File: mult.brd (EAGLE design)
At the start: 100 x 80 mm, 18 parts, among them IC1 TL074P

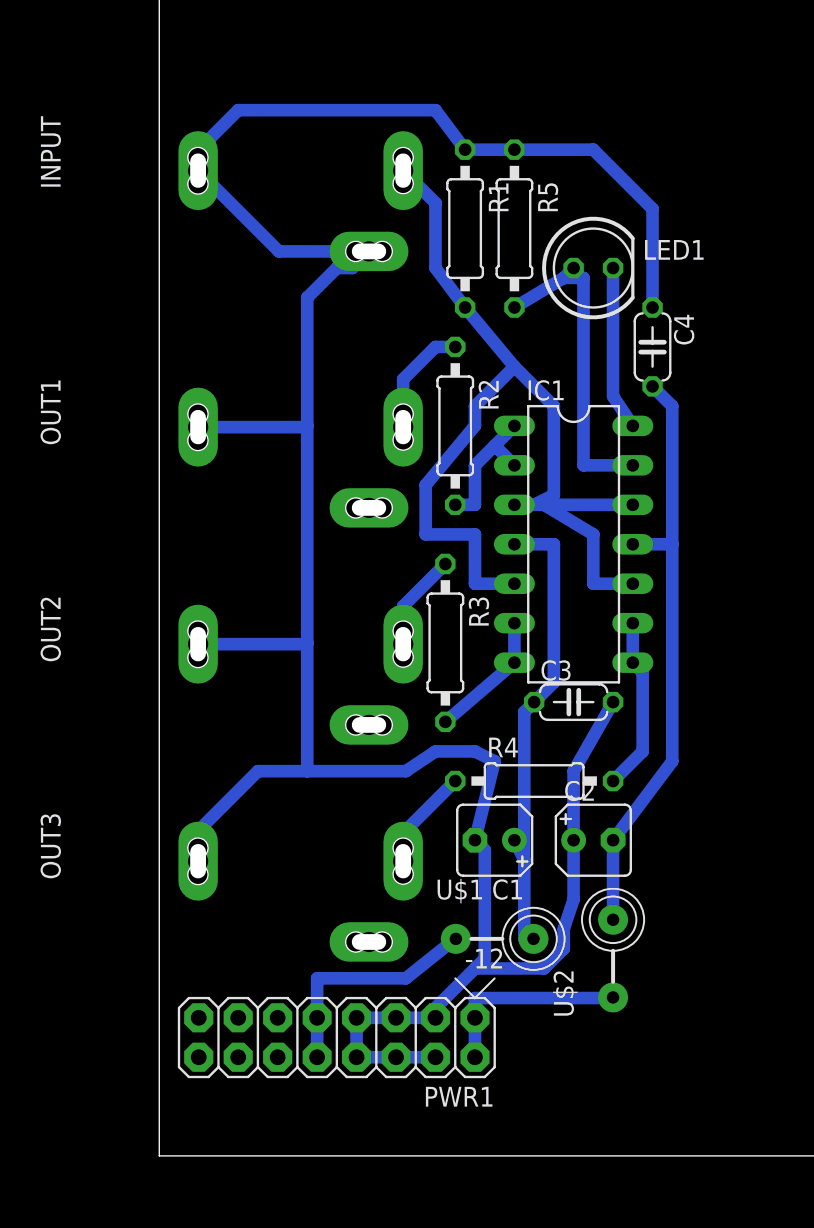
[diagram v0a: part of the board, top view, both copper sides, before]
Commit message: initial commit
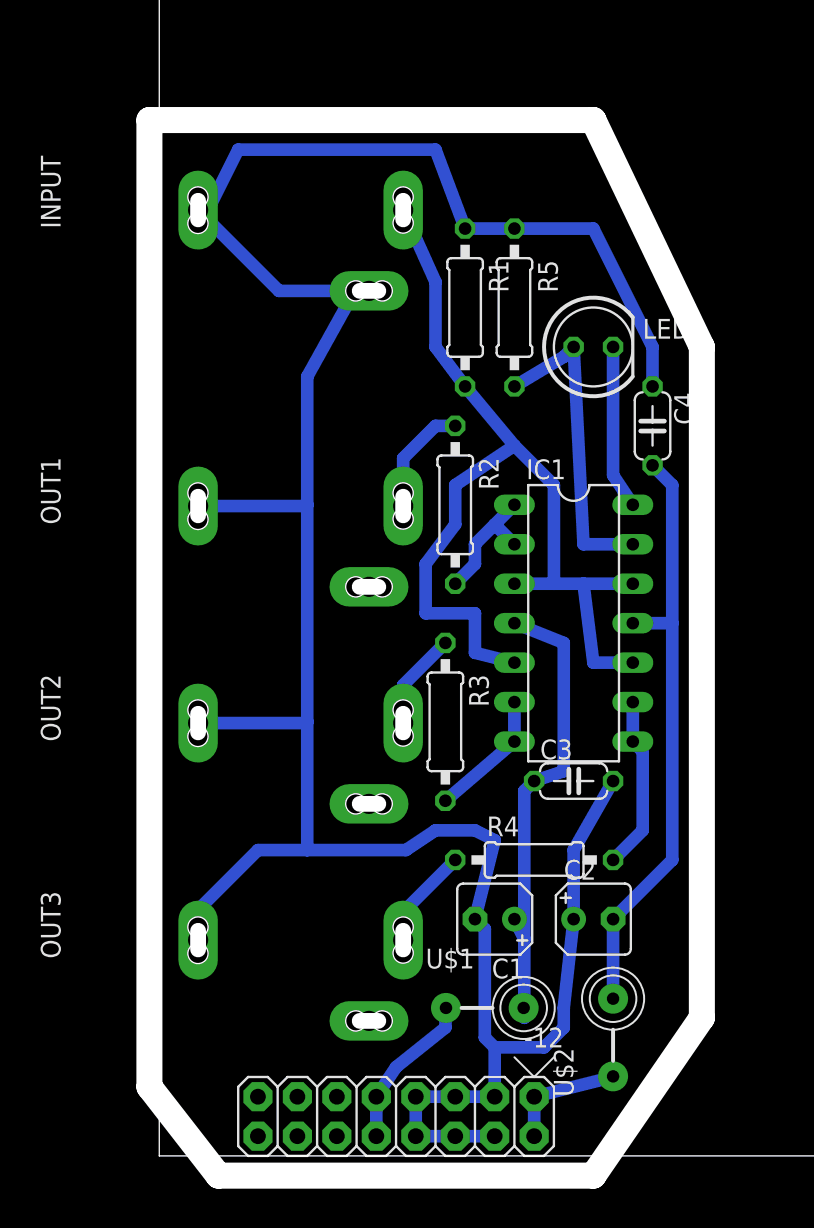
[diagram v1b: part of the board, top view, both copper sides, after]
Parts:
- moved PWR1 6.35 mm to (17.8, 2.54)
- moved R2 5.08 mm to (19.1, 41.9)
- moved C3 5.08 mm to (26.7, 24.1)
- moved OUT2 5.08 mm to (0.00, 22.9)
- moved R3 5.08 mm to (18.4, 27.9)
- moved C1 5.08 mm to (21.6, 15.2)
- moved C2 5.08 mm to (27.9, 15.2)
- moved OUT3 5.08 mm to (0.00, 8.89)
- moved U$2 5.08 mm to (29.2, 7.62)
- moved C4 5.08 mm to (31.8, 47.0)
- moved IC1 5.08 mm to (26.7, 34.3)
- moved LED1 5.08 mm to (27.9, 52.1)
- moved OUT1 5.08 mm to (0.00, 36.8)
- moved R1 5.08 mm to (19.7, 54.6)
- moved R4 5.08 mm to (24.1, 19.1)
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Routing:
- net N$2: track 12.7 -> 7.82 mm
- net N$1: track 14.9 -> 10.2 mm
- net GND: track 180.8 -> 184.6 mm
- net N$7: track 9.20 -> 8.45 mm
- net N$11: track 21.1 -> 20.5 mm
- net N$6: track 64.9 -> 64.4 mm
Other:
- board size 100 x 80 mm -> 100.6 x 81.3 mm
